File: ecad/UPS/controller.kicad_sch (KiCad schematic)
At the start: 32 parts, among them J2 Conn_01x05_Socket, SW1 SW_Push, SW2 SW_Push, U1 STM32L152RCT6, U2 AP2112K-3.3TRG1

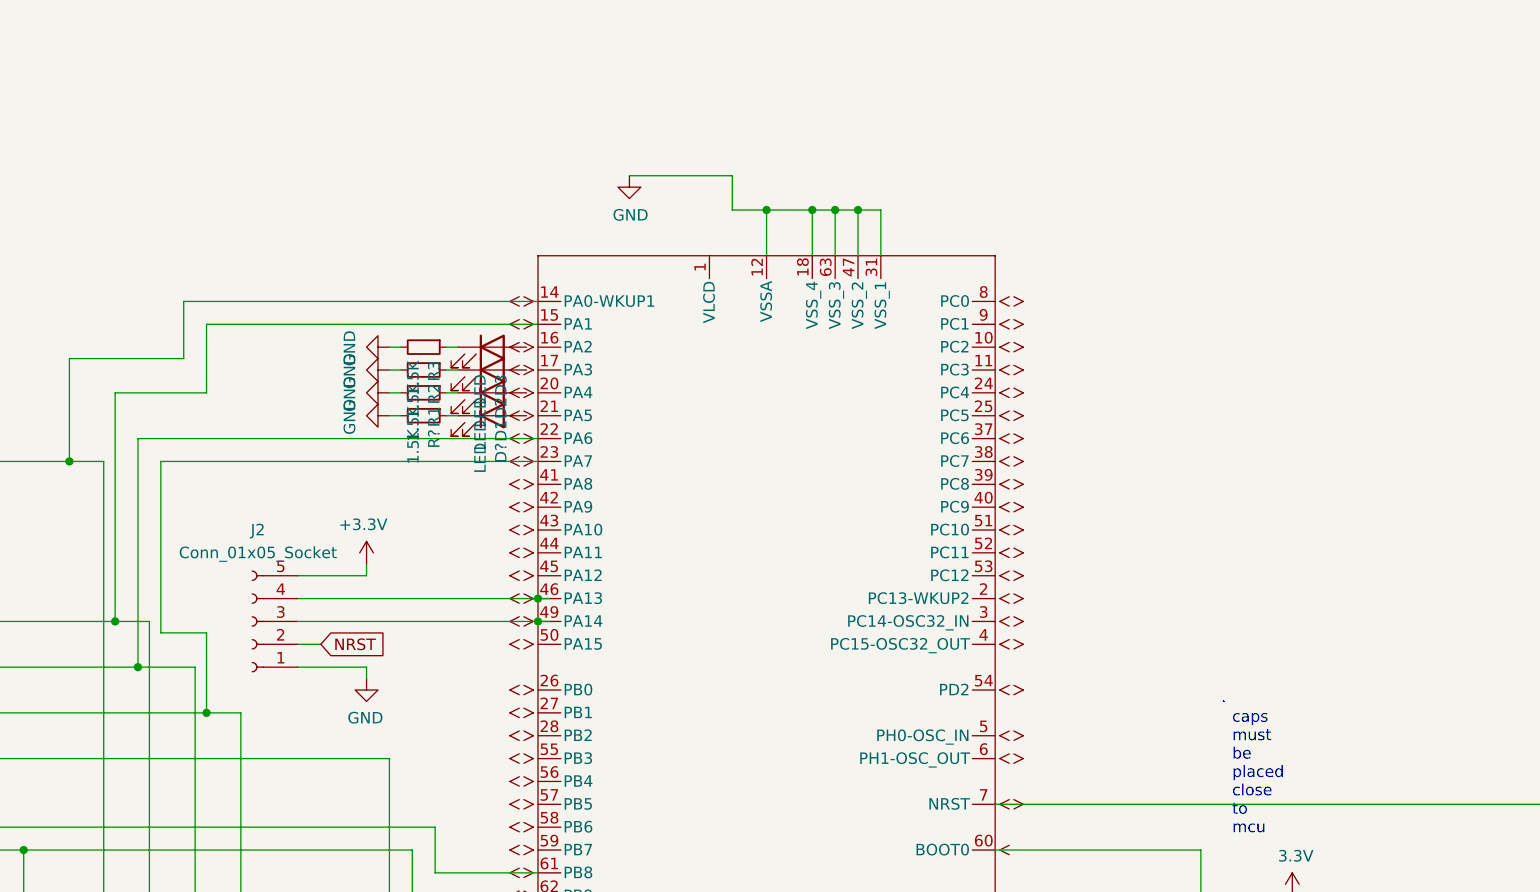
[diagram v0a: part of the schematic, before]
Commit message: minor things
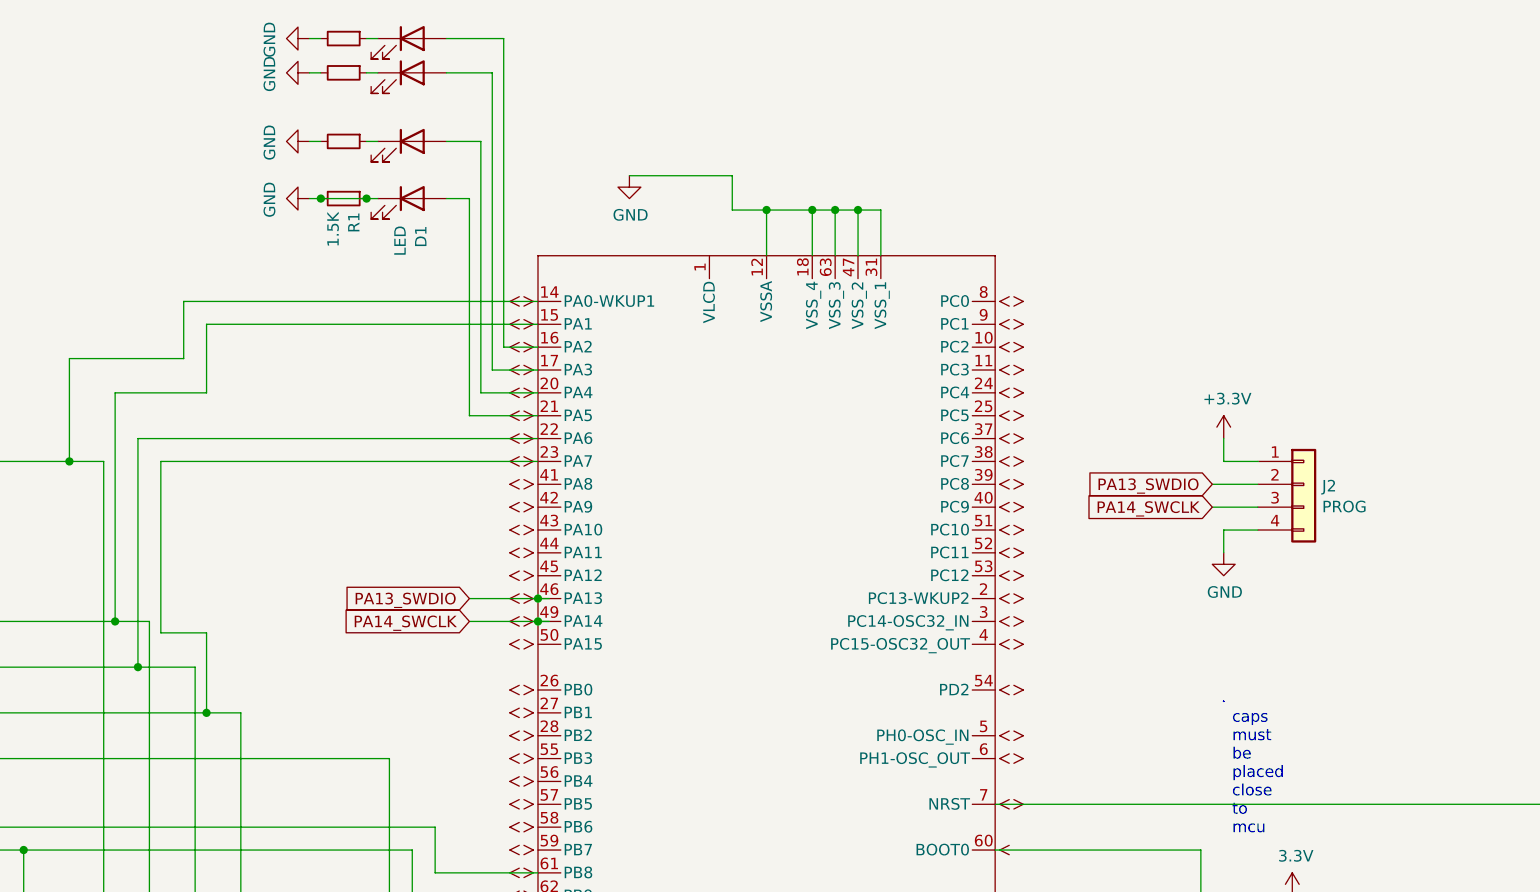
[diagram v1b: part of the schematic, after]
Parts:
- removed J2: Conn_01x05_Socket, symbol Connector:Conn_01x05_Socket
- added J2: PROG, Connector_PinHeader_2.54mm:PinHeader_1x04_P2.54mm_Vertical, symbol Connector_Generic:Conn_01x04
- gave numbers to parts that had none: 2
- renumbered D3 to D4, R3 to R4
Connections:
- net +3.3V: now also J2.1 (Pin_1)
- net GND: now also D1.1 (K), R1.1, J2.4 (Pin_4)
- net at D1.2 (A): now also U1.21 (PA5)
- net at D2.2 (A): now also U1.17 (PA3)
- net at D4.2 (A): now also U1.16 (PA2)
- net at D1.2 (A): now also U1.20 (PA4)
- net PA14_SWCLK: now reaches U1.49 (PA14)
- net PA14_SWCLK: now also J2.3 (Pin_3)
- net PA13_SWDIO: now reaches U1.46 (PA13)
- net PA13_SWDIO: now also J2.2 (Pin_2)
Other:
- moved on the sheet: D1, R1
